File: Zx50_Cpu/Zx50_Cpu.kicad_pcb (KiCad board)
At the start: 2 copper layers, 135.9 x 100.4 mm, 25 parts, among them J1 Zx50_EdgeConnector, J2 FrontPanelConnect, J20 Conn_02x05_Odd_Even, J3 Clock Mezzanine, J4 Front Panel, SW1 RESET, U1 74AHC1G14, U2 SN74AHCT245N, U3 SN74AHCT245N, U4 Z84C00xxP, U5 SN74AHCT245N, U6 MCP1316MT-46LE/OT, U7 SN74AHCT245N

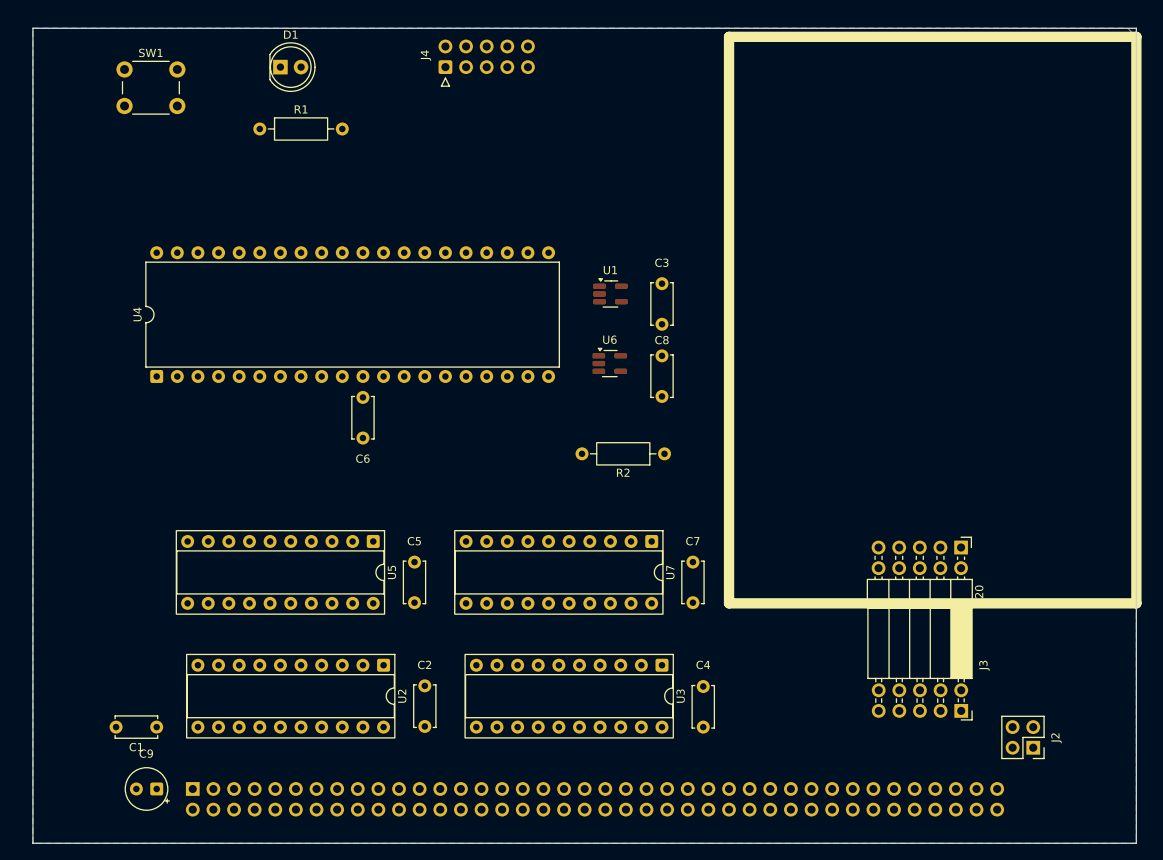
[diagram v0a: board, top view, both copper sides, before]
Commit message: 4 layer done
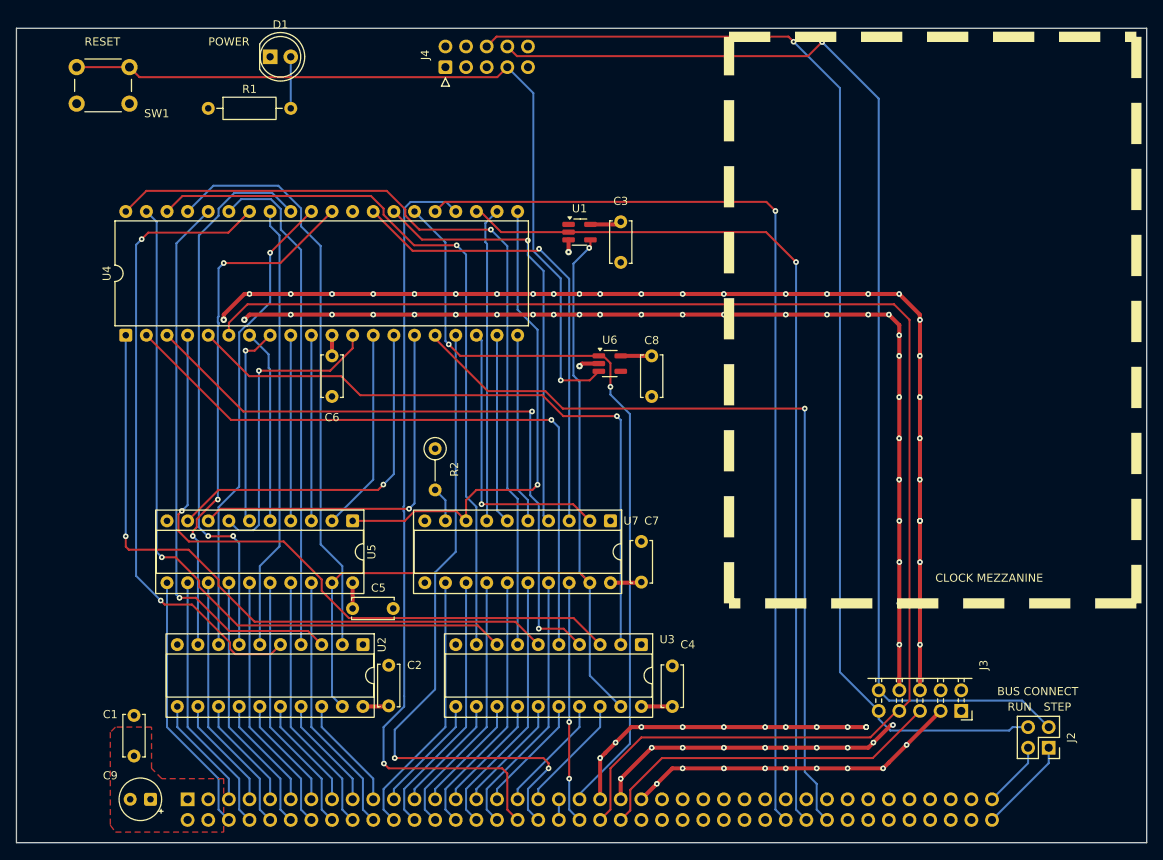
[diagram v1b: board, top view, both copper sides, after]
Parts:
- removed J20: Conn_02x05_Odd_Even, zx50_footprints:PinHeader_2x05_P2.54mm_Horizontal_Edge
- R2: footprint Resistor_THT:R_Axial_DIN0207_L6.3mm_D2.5mm_P10.16mm_Horizontal -> Resistor_THT:R_Axial_DIN0207_L6.3mm_D2.5mm_P5.08mm_Vertical
- moved R2 28.3 mm to (71.1, 115.6), turned to -90 degrees
- moved C3 9.16 mm to (94.0, 87.6)
- moved U1 8.52 mm to (88.9, 88.9)
- moved C5 7.65 mm to (61.0, 135.3), turned to 0 degrees
- moved C7 6.84 mm to (96.5, 132.0)
- moved R1 6.84 mm to (43.2, 73.7)
- moved C6 6.38 mm to (58.4, 104.1)
- moved U4 6.35 mm to (33.0, 101.6)
- moved SW1 5.90 mm to (27.0, 68.6)
- moved U7 5.68 mm to (92.7, 124.5)
- moved C2 5.12 mm to (65.4, 147.2)
- moved C4 4.58 mm to (100.3, 147.3)
- moved C1 4.52 mm to (34.0, 153.4), turned to 90 degrees
- moved U3 3.59 mm to (96.5, 139.7)
- moved U2 3.59 mm to (62.2, 139.7)
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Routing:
- net GND: track 0.00 -> 384.8 mm, vias 0 -> 89
- net /CLK: track 0.00 -> 181.7 mm
- net /~STEP: track 0.00 -> 145.5 mm, vias 0 -> 1
- net /RUN: track 0.00 -> 145.5 mm, vias 0 -> 1
- net /~BUSRQ~: track 0.00 -> 118.4 mm, vias 0 -> 1
- net /~BUSAK~: track 0.00 -> 110.7 mm, vias 0 -> 1
- net /BUSAK: track 0.00 -> 109.3 mm, vias 0 -> 1
- net /A10: track 0.00 -> 100.9 mm, vias 0 -> 1
- net /~INT~: track 0.00 -> 100.9 mm, vias 0 -> 1
- net /~RESET_SW: track 0.00 -> 100.5 mm, vias 0 -> 1
- net /~WAIT~: track 0.00 -> 98.6 mm, vias 0 -> 1
- net /~RESET~: track 0.00 -> 95.7 mm, vias 0 -> 2
- net /A8: track 0.00 -> 89.6 mm, vias 0 -> 1
- net /A9: track 0.00 -> 89.5 mm, vias 0 -> 1
- net /A14: track 0.00 -> 83.1 mm, vias 0 -> 1
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- added copper zone on F.Cu, net +5V
- added copper zone on In2.Cu, net +5V
- added copper zone on In1.Cu, net GND
- removed copper zone on B.Cu, net GND
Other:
- board size 135.9 x 100.4 mm -> 139.2 x 100.3 mm
- copper layers 2 -> 4
- board text added: "BUS CONNECT"
- board text added: "CLOCK MEZZANINE"
- board text added: "POWER"
- board text added: "RESET"
- board text added: "RUN"
- board text added: "STEP"
